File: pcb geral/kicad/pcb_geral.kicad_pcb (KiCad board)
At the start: 2 copper layers, 138 x 57 mm, 7 parts

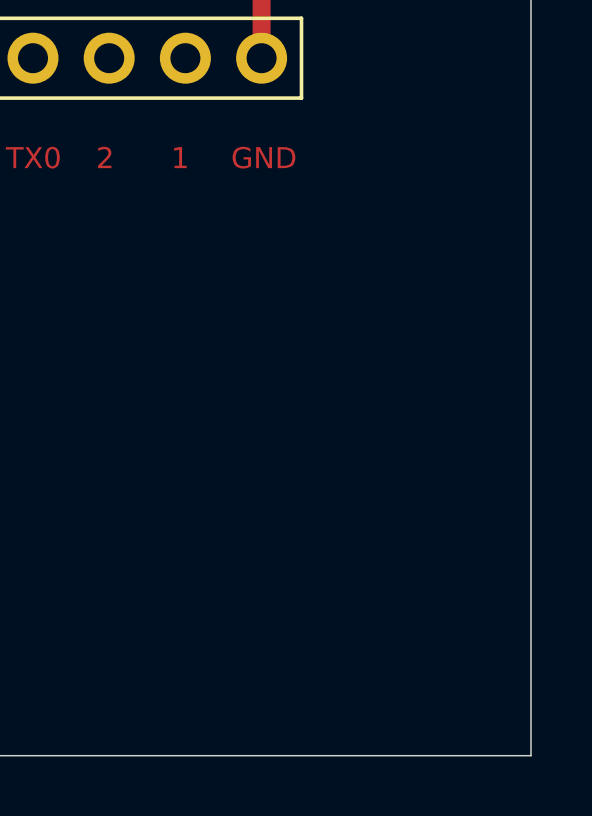
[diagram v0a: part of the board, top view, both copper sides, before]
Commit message: Backup
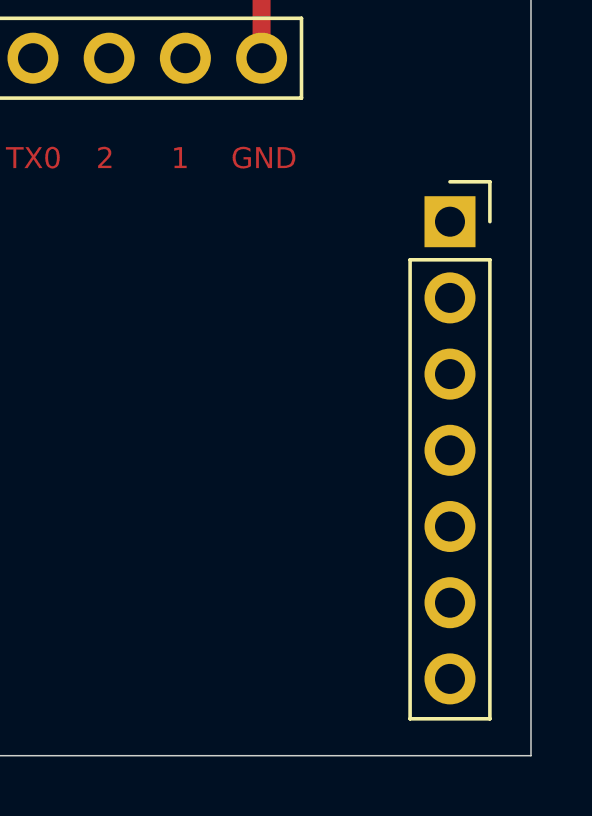
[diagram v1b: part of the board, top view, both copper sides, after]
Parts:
- added REF**: PinSocket_1x07_P2.54mm_Vertical, Connector_PinSocket_2.54mm:PinSocket_1x07_P2.54mm_Vertical, F.Cu at (214.8, 115.2)
